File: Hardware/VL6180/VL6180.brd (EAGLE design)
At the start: 160 x 100 mm, 28 parts, among them T1 2N7002BKS, T2 2N7002BKS, U1 VL6180X, U2 VL6180X, U3 MIC5225_2.8V

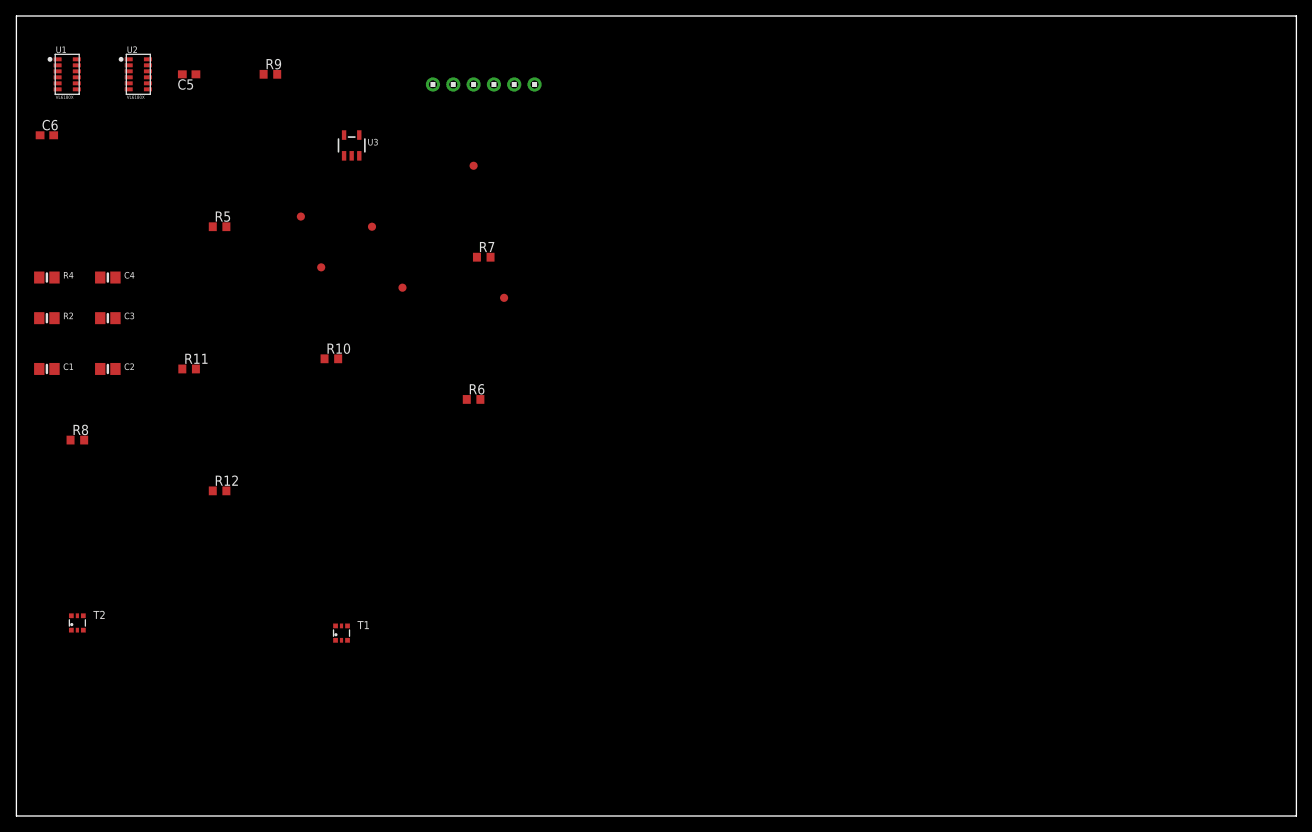
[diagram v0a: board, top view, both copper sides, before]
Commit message: update 02-10-2017
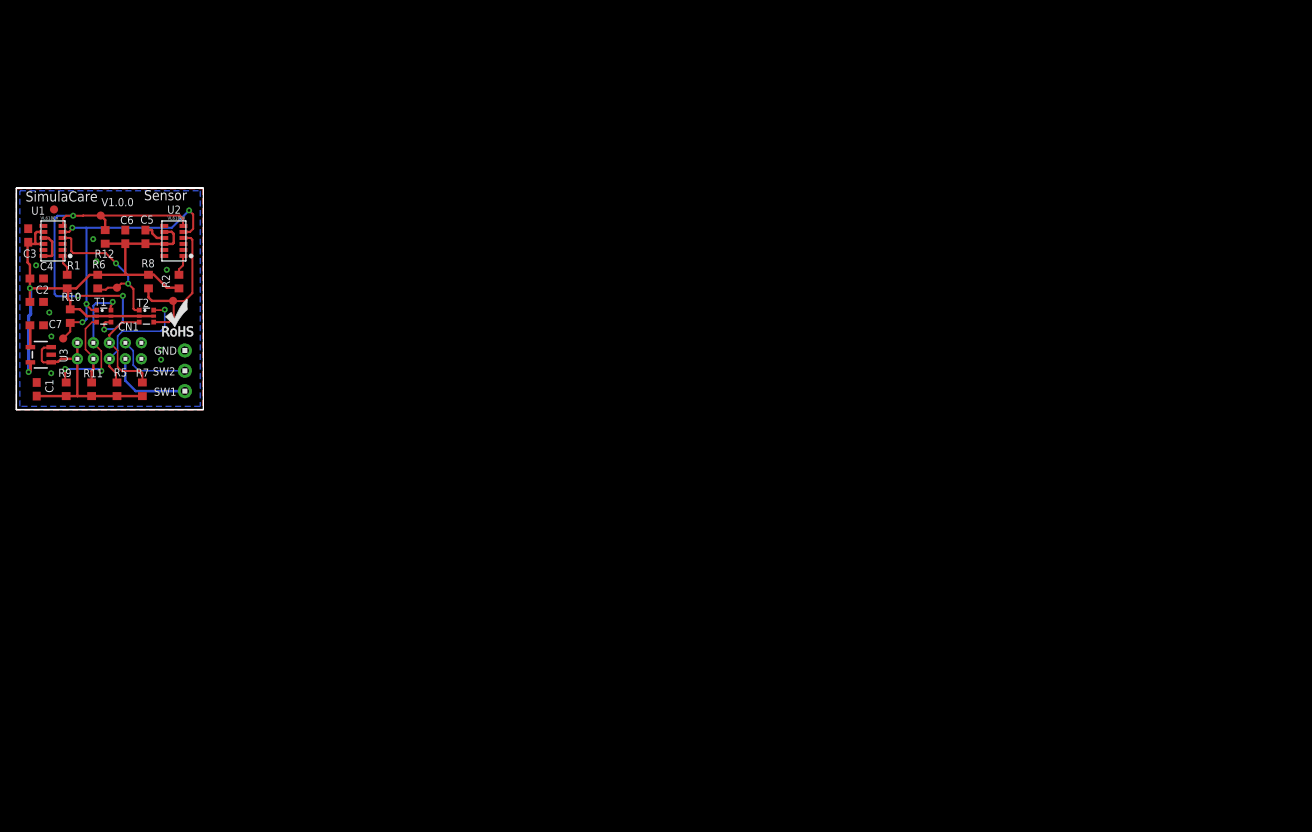
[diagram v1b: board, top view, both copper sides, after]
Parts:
- removed R4: 47K, microbuilder:0805-NO
- removed TP6: GPIO1-0, SparkFun-Connectors:PAD.03X.04
- added C7: 470pF, resistor:C0603
- added R1: 47K, resistor:R0603
- added U$20: (no value), SparkFun-Aesthetics:ROHS_LOGO_0.18_IN
- added U$3: 2X5, headers(2mm)(samtec):2X5
- C1: value 0.1uF -> 1uF; device microbuilder:0805-NO -> resistor:C0603
- C2: value 0.1uF -> 10uF; device microbuilder:0805-NO -> resistor:C0603
- C3: value 10uF -> 100nF; device microbuilder:0805-NO -> resistor:C0603
- C4: value 10uF -> 4.7uF; device microbuilder:0805-NO -> resistor:C0603
- C5: value 4.7uF -> 100nF; device rcl:C0603 -> resistor:C0603
- C6: device rcl:C0603 -> resistor:C0603
- H1: value 1X6 -> 1X3; device header:1X6 -> headers(.1in):1X3
- R2: device microbuilder:0805-NO -> resistor:R0603
- T1, T2: value 2N7002BKS -> 2N7002DW
- TP1: value SDA -> SCL
- TP2: value SCL -> SDA
- TP5: value GPIO1-1 -> GND
- U3: value MIC5225_2.8V -> MIC5219_2.8V
- moved TP1 55.4 mm to (5.84, 59.7)
- moved T1 49.5 mm to (10.9, 62.5), turned to 270 degrees
- moved H1 49.3 mm to (21.1, 53.1), turned to 90 degrees
- moved R6 49.2 mm to (10.2, 66.8), turned to 270 degrees
- moved R9 46.9 mm to (6.22, 53.3), turned to 90 degrees
- moved U3 46.8 mm to (3.05, 57.7), turned to 90 degrees
- moved R7 45.8 mm to (15.7, 53.3), turned to 90 degrees
- moved T2 39.3 mm to (16.3, 62.5), turned to 270 degrees
- moved TP2 38.8 mm to (10.5, 75.1)
- moved R12 34.8 mm to (11.1, 72.4), turned to 90 degrees
- moved R10 33.1 mm to (6.73, 62.5), turned to 270 degrees
- moved TP3 32.8 mm to (12.6, 66.0)
- moved TP5 30.9 mm to (4.70, 75.8)
- moved R5 24.0 mm to (12.6, 53.3), turned to 90 degrees
- moved R8 21.7 mm to (16.5, 66.8), turned to 270 degrees
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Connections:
- new net N$2: C7.1, U3.4
- new net SW1: H1.1, U$3.7
- new net SW2: H1.2, U$3.8
- net 2.8V: now also C2.1, C4.1, R1.2; no longer C1.2, C2.2, R4.2
- net 3.3V: now also C1.1, U$3.1, U$3.2; no longer C4.1, H1.1
- net CS0: now also U$3.5; no longer H1.4
- net CS1: now also U$3.6; no longer H1.5
- net GND: now also C1.2, C2.2, C7.2, H1.3, TP5.P$1, U$3.10, U$3.9; no longer C1.1, C2.1, H1.6
- net N$1: now also R1.1; no longer R2.1, TP6.P$1
- net N$3: now also R2.1; no longer R4.1, TP5.P$1
- net SCL: now also U$3.4; no longer H1.3
- net SDA: now also U$3.3; no longer H1.2
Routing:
- net 2.8V: track 0.00 -> 73.3 mm, vias 0 -> 2
- net N$9: track 0.00 -> 47.5 mm, vias 0 -> 4
- net N$5: track 0.00 -> 38.5 mm, vias 0 -> 4
- net 3.3V: track 0.00 -> 27.3 mm
- net CS0_LV: track 0.00 -> 20.5 mm, vias 0 -> 2
- net CS1_LV: track 0.00 -> 20.0 mm
- net SCL: track 0.00 -> 18.8 mm, vias 0 -> 3
- net CS0: track 0.00 -> 16.6 mm, vias 0 -> 1
- net CS1: track 0.00 -> 13.4 mm
- net SW1: track 0.00 -> 10.7 mm
- net SW2: track 0.00 -> 9.94 mm
- net SDA: track 0.00 -> 8.95 mm
- net GND: track 0.00 -> 7.07 mm, vias 0 -> 9
- net N$2: track 0.00 -> 2.99 mm
- net N$1: track 0.00 -> 2.59 mm
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- added copper zone on layer 1, net GND
- added copper zone on layer 16, net GND
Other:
- board size 160 x 100 mm -> 23.4 x 27.7 mm
- board text added: "CN1"
- board text added: "GND"
- board text added: "SW1"
- board text added: "SW2"
- board text added: "Sensor"
- board text added: "SimulaCare"
- board text added: "V1.0.0"
